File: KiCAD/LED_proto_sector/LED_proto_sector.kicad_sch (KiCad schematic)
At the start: 6 parts, among them J2 PJ-082BH

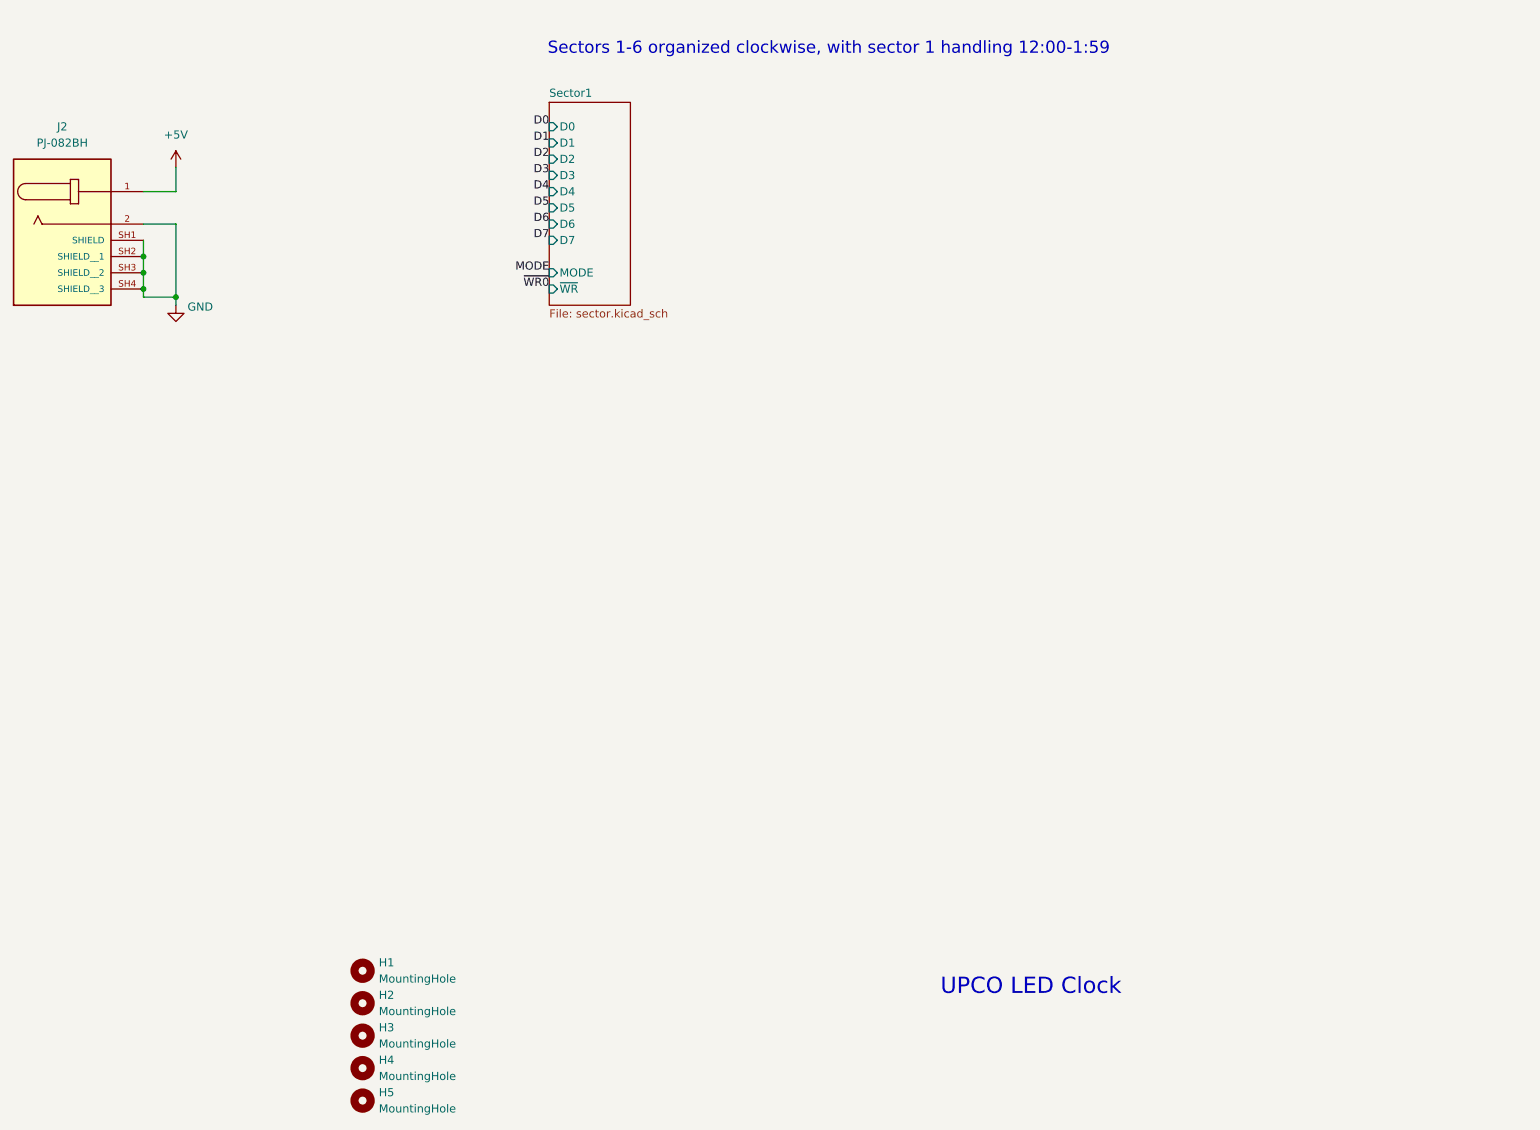
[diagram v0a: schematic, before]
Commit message: prototype sector
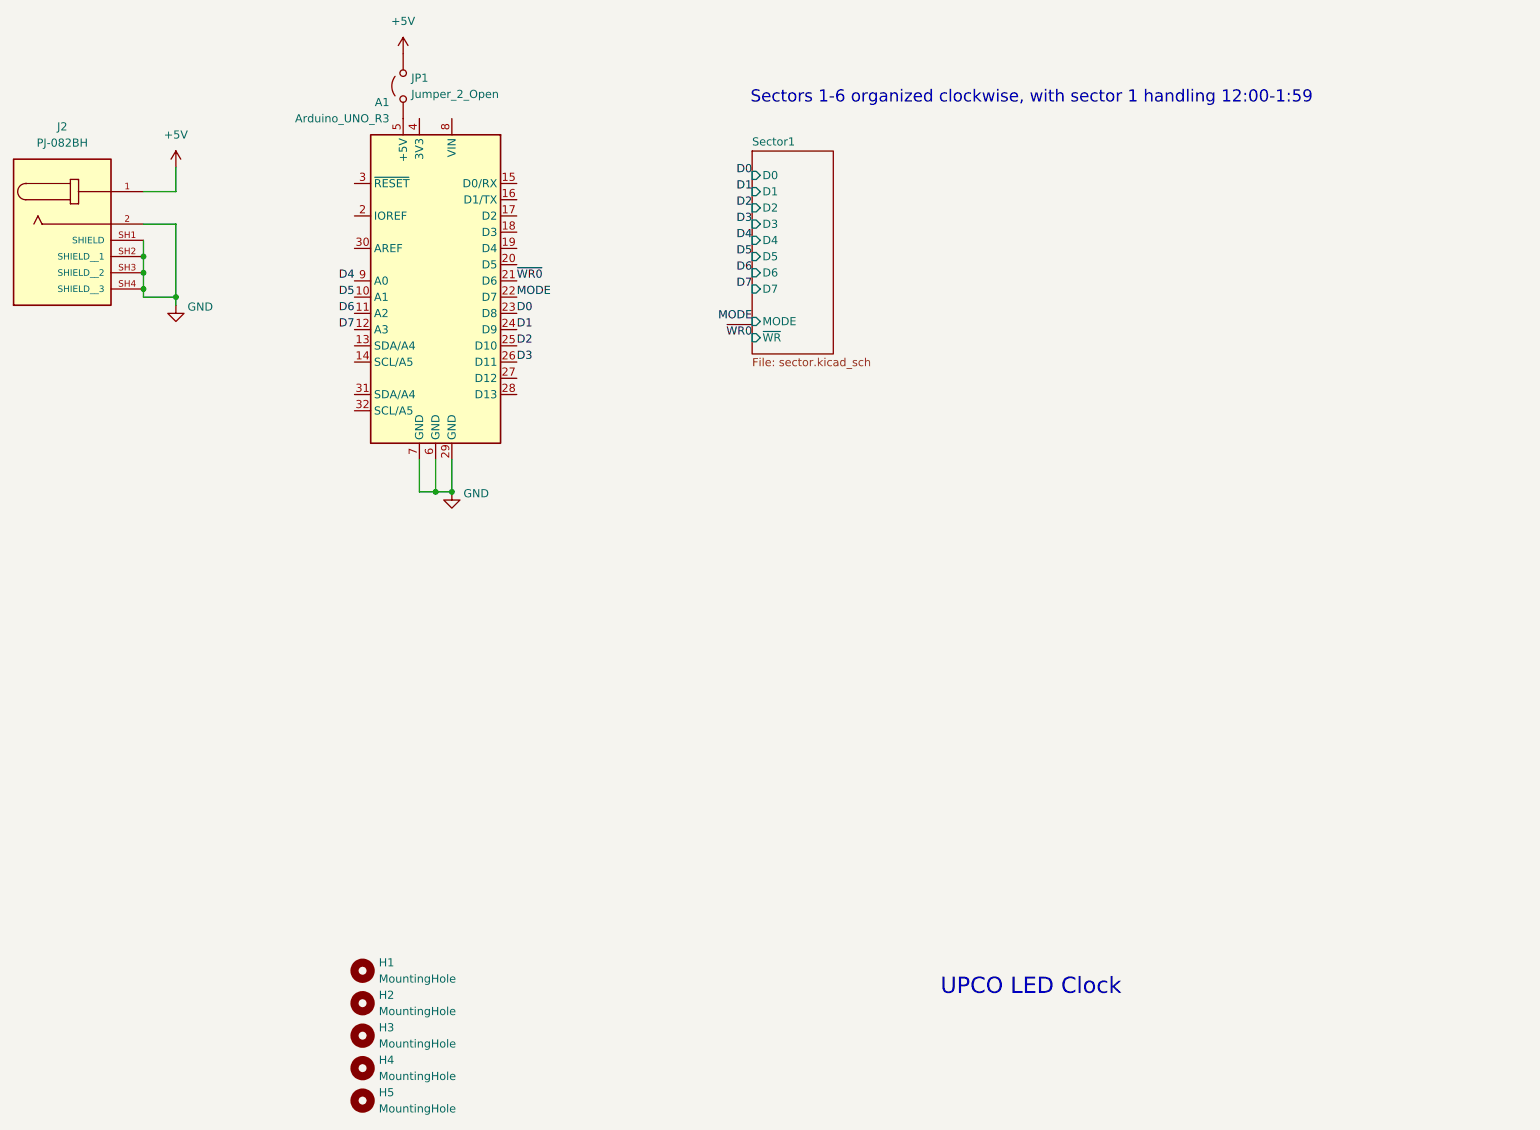
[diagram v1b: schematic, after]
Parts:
- added A1: Arduino_UNO_R3, Module:Arduino_UNO_R3, symbol MCU_Module:Arduino_UNO_R3
- added JP1: Jumper_2_Open, Connector_PinHeader_2.54mm:PinHeader_1x02_P2.54mm_Vertical, symbol Jumper:Jumper_2_Open
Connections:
- net +5V: now also JP1.2 (B)
- net D0: now also A1.23 (D8)
- net D1: now also A1.24 (D9)
- net D2: now also A1.25 (D10)
- net D3: now also A1.26 (D11)
- net D4: now also A1.9 (A0)
- net D5: now also A1.10 (A1)
- net D6: now also A1.11 (A2)
- net D7: now also A1.12 (A3)
- net GND: now also A1.29 (GND), A1.6 (GND), A1.7 (GND)
- net MODE: now also A1.22 (D7)
- net ~{WR0}: now also A1.21 (D6)
- new net: A1.5 (+5V), JP1.1 (A)
